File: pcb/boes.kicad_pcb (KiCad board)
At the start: 2 copper layers, 18 parts, among them J1 SW_A, J10 HUB75 Display ctrl, J2 SW_B, J3 SW_C, J4 Pot_J, J5 Pot_P, J6 Sens_J, J7 Sens_P, J8 Buzzer, J9 Display power, Q1 2N7000, U1 PicoW

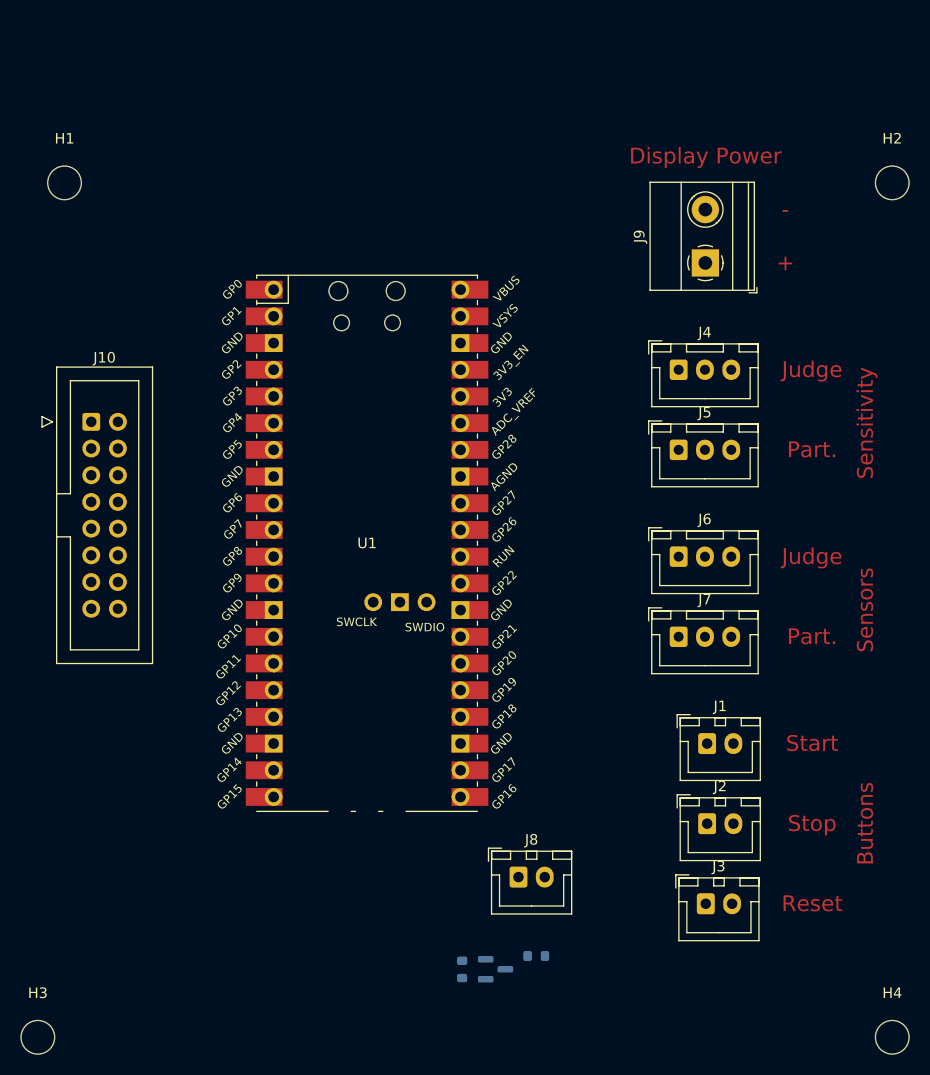
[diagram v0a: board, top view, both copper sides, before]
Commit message: Main PCB ready for final tweaks
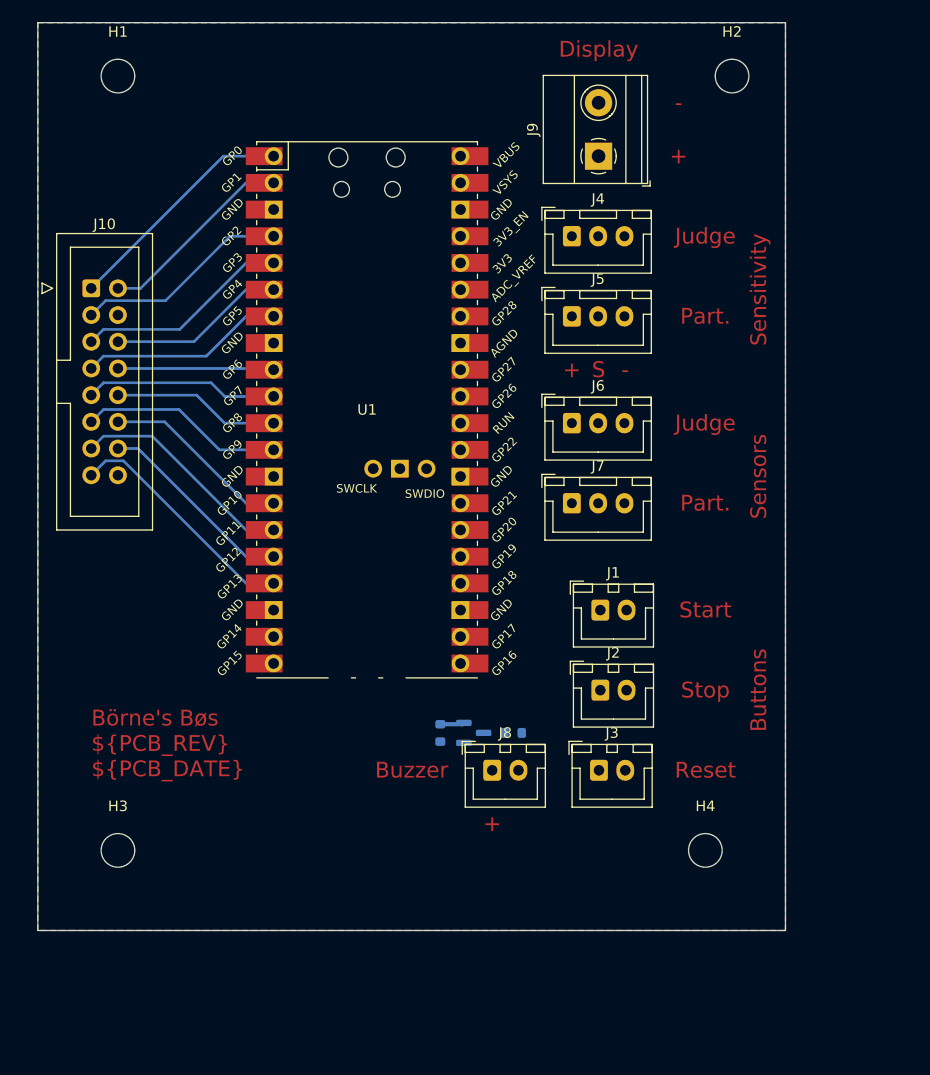
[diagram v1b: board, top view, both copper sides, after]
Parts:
- moved H4 25.1 mm to (157.5, 129.5)
- moved Q1 22.6 mm to (135.4, 118.4)
- moved R1 22.6 mm to (132.3, 118.4)
- moved R2 21.3 mm to (139.2, 118.4)
- moved H3 19.3 mm to (101.6, 129.5)
- moved H2 18.3 mm to (160.0, 55.9)
- moved J2 16.3 mm to (147.5, 114.3)
- moved J3 16.3 mm to (147.4, 121.9)
- moved J5 16.3 mm to (144.8, 78.7)
- moved J7 16.3 mm to (144.8, 96.5)
- moved J1 16.3 mm to (147.5, 106.7)
- moved J4 16.3 mm to (144.8, 71.1)
- moved J6 16.3 mm to (144.8, 88.9)
- moved J9 14.4 mm to (147.3, 63.5)
- moved J10 12.7 mm to (99.1, 76.1)
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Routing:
- net OE: track 0.00 -> 22.7 mm
- net R1: track 0.00 -> 22.6 mm
- net CLK: track 0.00 -> 21.5 mm
- net R2: track 0.00 -> 20.5 mm
- net B1: track 0.00 -> 20.5 mm
- net C: track 0.00 -> 19.4 mm
- net B2: track 0.00 -> 19.4 mm
- net Latch: track 0.00 -> 19.1 mm
- net G1: track 0.00 -> 19.0 mm
- net A: track 0.00 -> 18.4 mm
- net D: track 0.00 -> 18.0 mm
- net G2: track 0.00 -> 16.9 mm
- net B: track 0.00 -> 15.9 mm
- net E: track 0.00 -> 14.9 mm
- net Buzzer: track 0.00 -> 2.51 mm
- added copper zone on F.Cu, net (none)
- added copper zone on B.Cu, net GND
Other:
- board outline added: 71.1 x 86.4 mm
- board text added: "Buzzer"
- board text added: "Börne's Bøs ${PCB_REV} ${PCB_DATE}"
- board text added: "Display"
- board text added: "S"
- board text removed: "Display Power"
